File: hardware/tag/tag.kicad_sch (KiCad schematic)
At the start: 8 parts

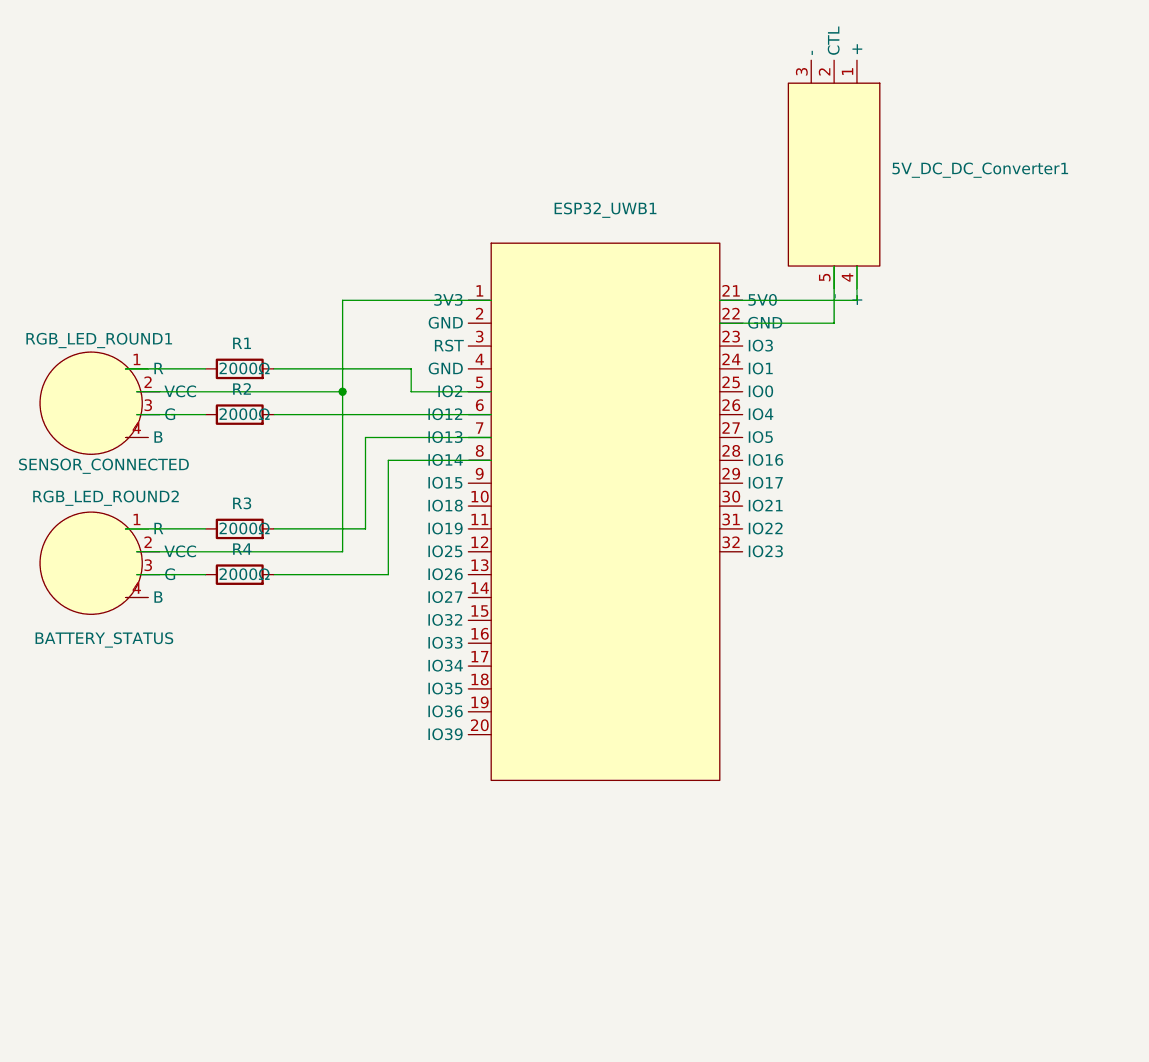
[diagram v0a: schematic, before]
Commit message: hardware: Add remote PCB.
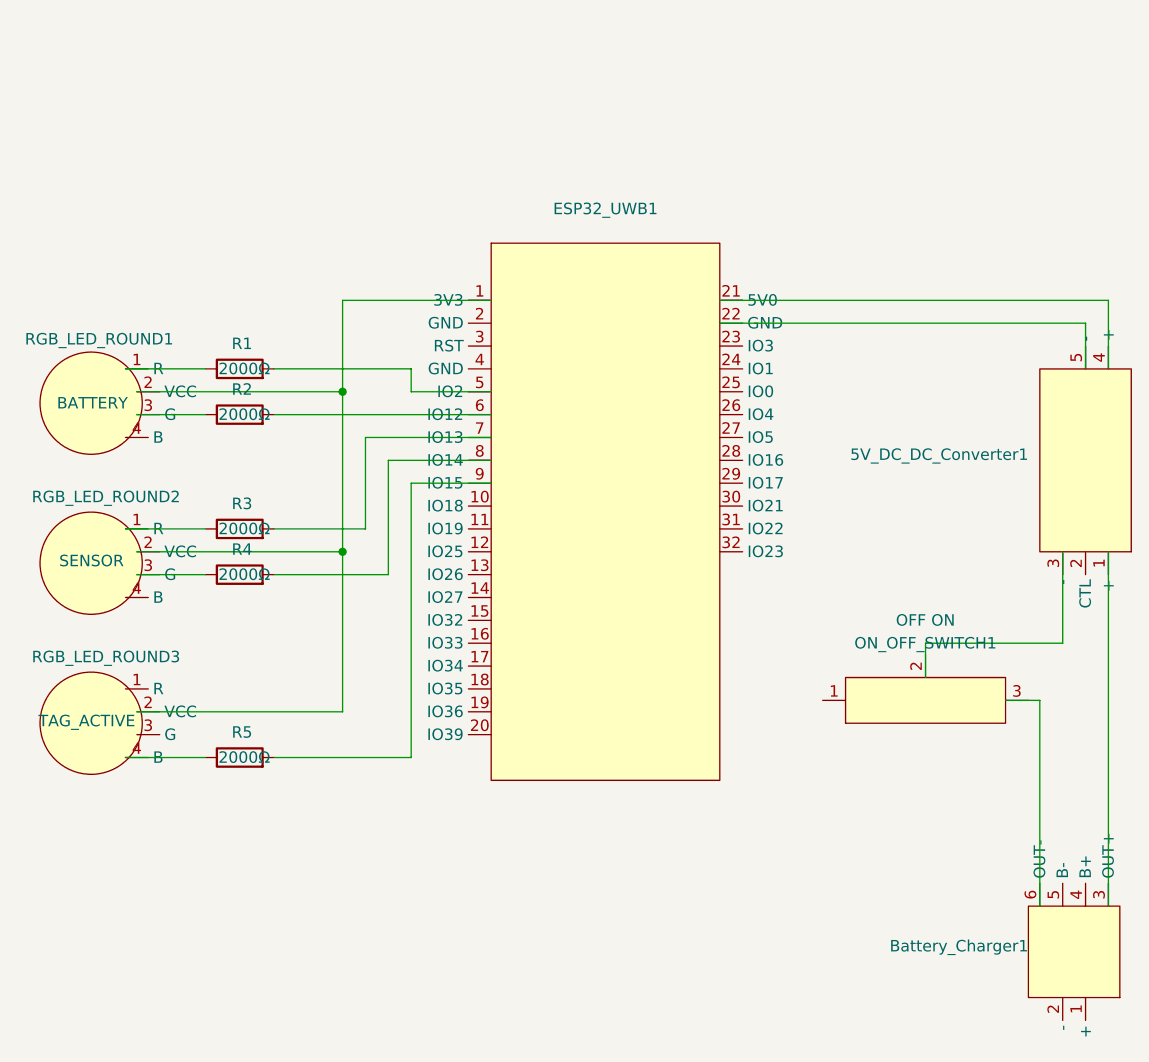
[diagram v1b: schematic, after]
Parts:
- added Battery_Charger1: ~, Autocam:USB-C 3.7V Lithium Battery Charger, symbol Autocam:USB-C_3.7V_Lithium_Battery_Charger
- added ON_OFF_SWITCH1: OFF ON, Autocam:3-PIN Switch, symbol Autocam:3_PIN_Switch
- added R5: 2000Ω, Autocam:Simple Resistor, symbol Autocam:Simple Resistor
- added RGB_LED_ROUND3: TAG_ACTIVE, Autocam:Anode RGB LED (Round), symbol Autocam:ANODE_RGB_LED_Round
- RGB_LED_ROUND1: value SENSOR_CONNECTED -> BATTERY
- RGB_LED_ROUND2: value BATTERY_STATUS -> SENSOR
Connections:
- net at ESP32_UWB1.1 (3V3), RGB_LED_ROUND1.2 (VCC), RGB_LED_ROUND2.2 (VCC): now also RGB_LED_ROUND3.2 (VCC)
- net at ESP32_UWB1.9 (IO15): now also R5.2
- net at 5V_DC_DC_Converter1.1 (+): now also Battery_Charger1.3 (OUT+)
- net at 5V_DC_DC_Converter1.3 (-): now also ON_OFF_SWITCH1.2
- new net: R5.1, RGB_LED_ROUND3.4 (B)
- new net: Battery_Charger1.6 (OUT-), ON_OFF_SWITCH1.3
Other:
- moved on the sheet: 5V_DC_DC_Converter1
